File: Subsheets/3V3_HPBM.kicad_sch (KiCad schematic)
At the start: 8 parts, among them Q3 BSS123NH6327XTSA1

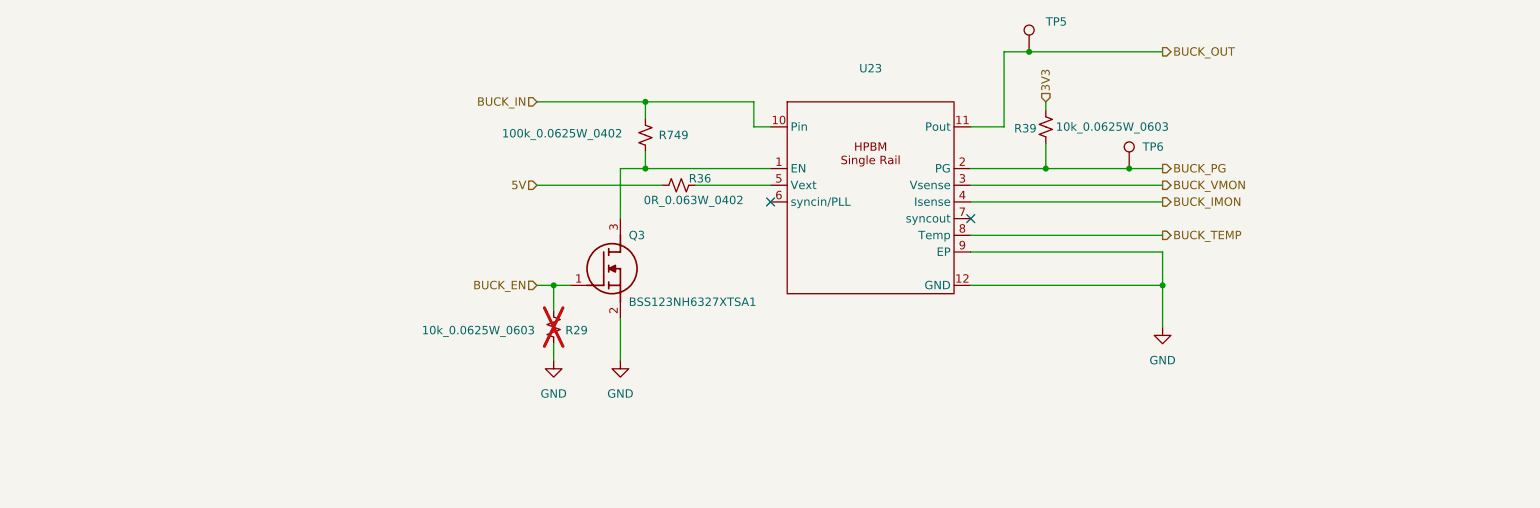
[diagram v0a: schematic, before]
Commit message: Schematic Update 1.2
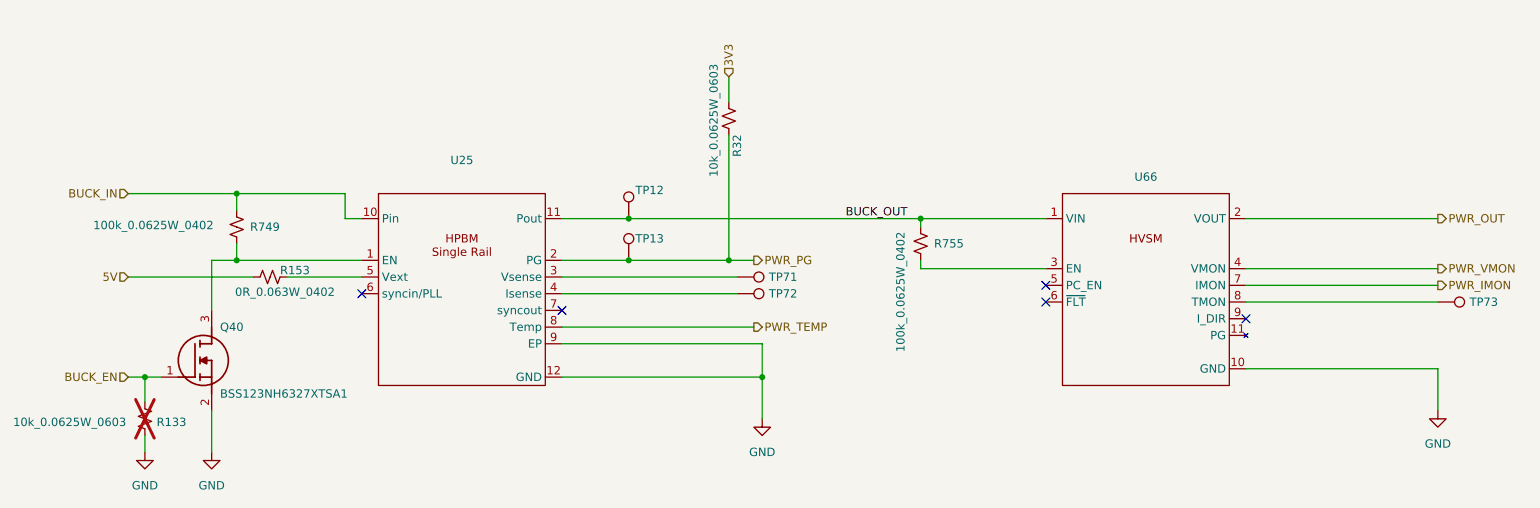
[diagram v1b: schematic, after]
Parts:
- removed Q3: BSS123NH6327XTSA1, SOT95P240X110-3N, symbol BSS123NH6327XTSA1:BSS123NH6327XTSA1
- removed R29, R39: 10k_0.0625W_0603, Pixxel_Resistors:RES0603, symbol Device:R_Small_US
- removed R36: 0R_0.063W_0402, Pixxel_Resistors:RES0402, symbol Device:R_Small_US
- removed TP5, TP6: TestPoint, symbol Connector:TestPoint
- removed U23: (no value), symbol Non-Isolated-Buck-Module_v9:HPBM_single_rail
- added Q40: BSS123NH6327XTSA1, SOT95P240X110-3N, symbol BSS123NH6327XTSA1:BSS123NH6327XTSA1
- added R133, R32: 10k_0.0625W_0603, Pixxel_Resistors:RES0603, symbol Device:R_Small_US
- added R153: 0R_0.063W_0402, Pixxel_Resistors:RES0402, symbol Device:R_Small_US
- added R755: 100k_0.0625W_0402, Pixxel_Resistors:RES0402, symbol Device:R_Small_US
- added TP12, TP13, TP71, TP72, TP73: TestPoint, symbol Connector:TestPoint
- added U25: (no value), symbol Non-Isolated-Buck-Module_v9:HPBM_single_rail
- added U66: (no value), symbol HVSM_LVSM_v9:HVSM
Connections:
- net 3V3: now also R32.1
- net 5V: now also R153.2
- net BUCK_EN: now also Q40.1 (G), R133.1
- net BUCK_IN: now also U25.10 (Pin)
- net BUCK_OUT: now also R755.2, TP12.1, U25.11 (Pout), U66.1 (VIN)
- net GND: now also Q40.2 (S), R133.2, U25.12 (GND), U25.9 (EP), U66.10 (GND)
- net at R749.1: now also Q40.3 (D), U25.1 (EN)
- new net: TP71.1, U25.3 (Vsense)
- new net: TP72.1, U25.4 (Isense)
- new net: R153.1, U25.5 (Vext)
- new net: R755.1, U66.3 (EN)
- new net: TP73.1, U66.8 (TMON)
- new net PWR_IMON: U66.7 (IMON)
- new net PWR_OUT: U66.2 (VOUT)
- new net PWR_PG: R32.2, TP13.1, U25.2 (PG)
- new net PWR_TEMP: U25.8 (Temp)
- new net PWR_VMON: U66.4 (VMON)
- no-connect marks 2 -> 5
